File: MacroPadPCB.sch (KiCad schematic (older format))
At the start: 24 parts, among them SW1 SW_Push, U1 ATmega32U4-AU, Y1 16MHz

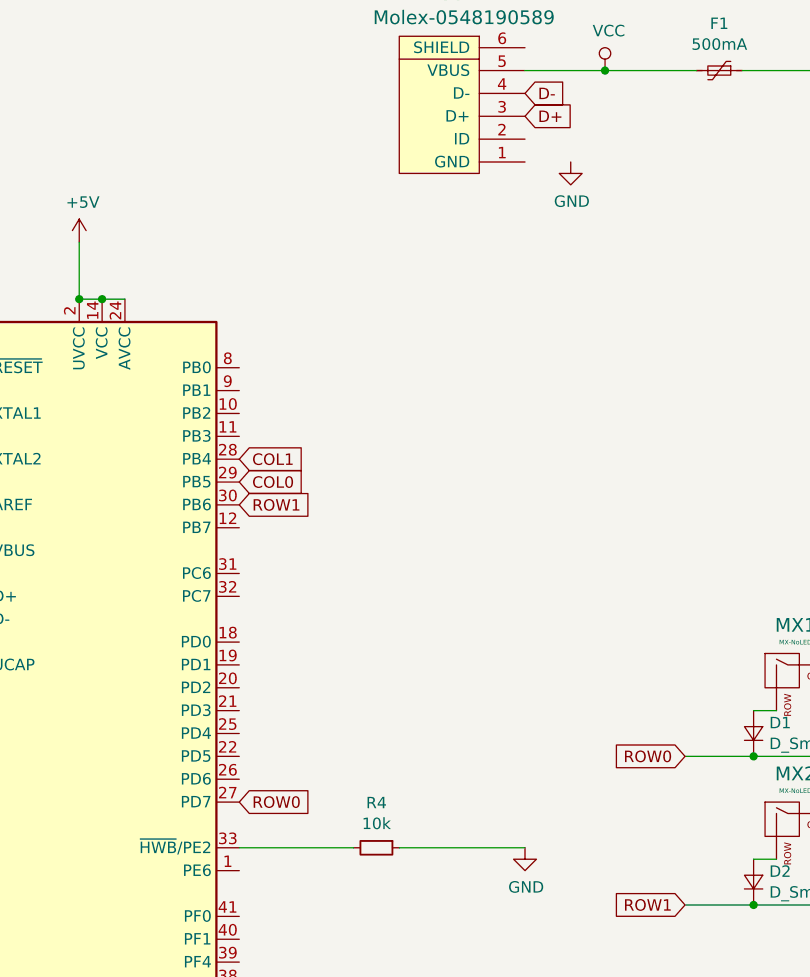
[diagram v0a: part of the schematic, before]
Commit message: PCB build and routing
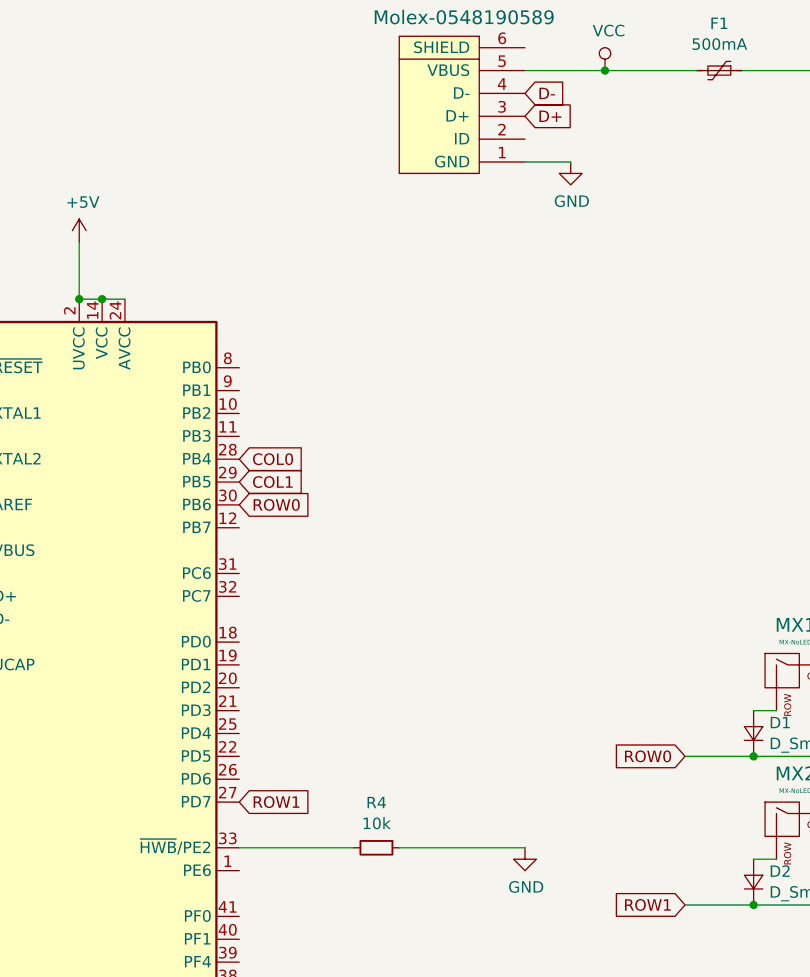
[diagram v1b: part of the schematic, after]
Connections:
- net COL0: now also U1.28 (PB4); no longer U1.29 (PB5)
- net COL1: now also U1.29 (PB5); no longer U1.28 (PB4)
- net GND: now also USB1.1 (GND)
- net ROW0: now also U1.30 (PB6); no longer U1.27 (PD7)
- net ROW1: now also U1.27 (PD7); no longer U1.30 (PB6)
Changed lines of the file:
@@
 Text GLabel 7100 4100 1    50   Input ~ 0
 COL1
+Text GLabel 3900 3650 2    50   Input ~ 0
+COL1
 Text GLabel 3900 3550 2    50   Input ~ 0
-COL1
-Text GLabel 3900 3650 2    50   Input ~ 0
 COL0
+Text GLabel 3900 5050 2    50   Input ~ 0
+ROW1
 Text GLabel 3900 3750 2    50   Input ~ 0
-ROW1
-Text GLabel 3900 5050 2    50   Input ~ 0
 ROW0
+Wire Wire Line
+	5150 2250 5350 2250
 $EndSCHEMATC
